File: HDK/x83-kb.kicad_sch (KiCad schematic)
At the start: 172 parts, among them U101 STM32F072C8Tx, U102 AMS1117-3.3

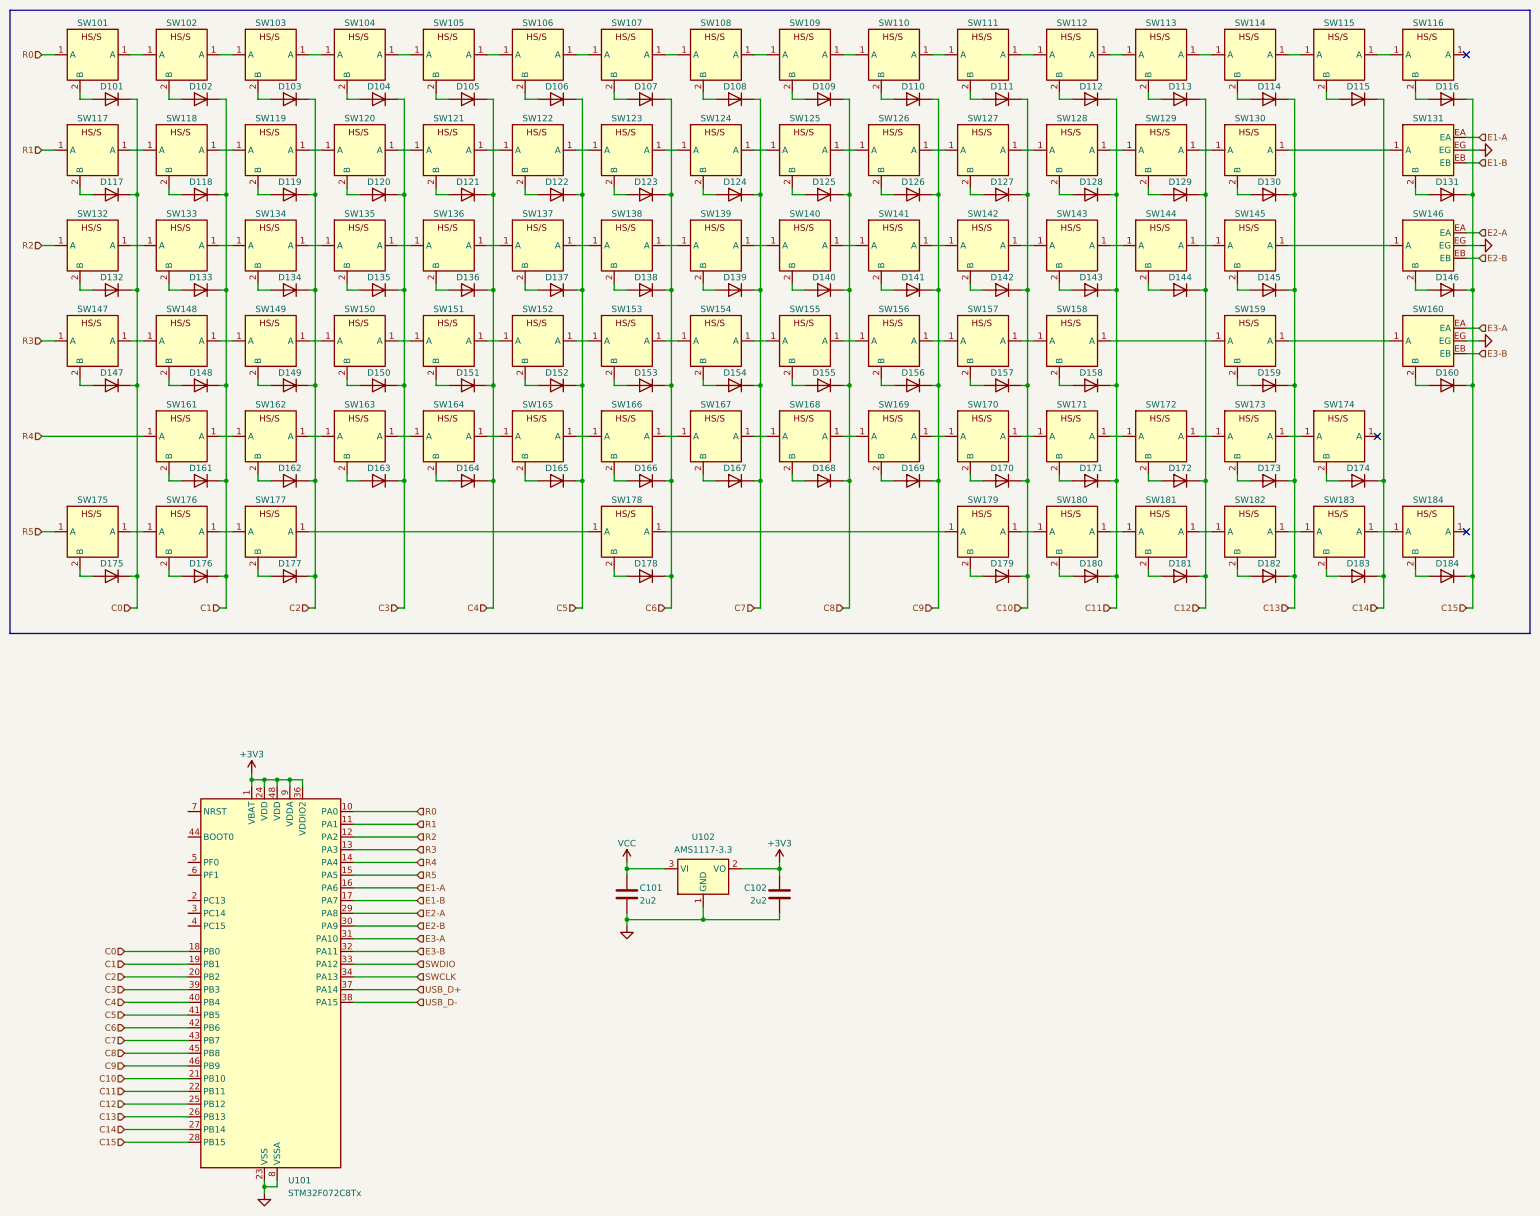
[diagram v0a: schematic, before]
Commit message: added rsc
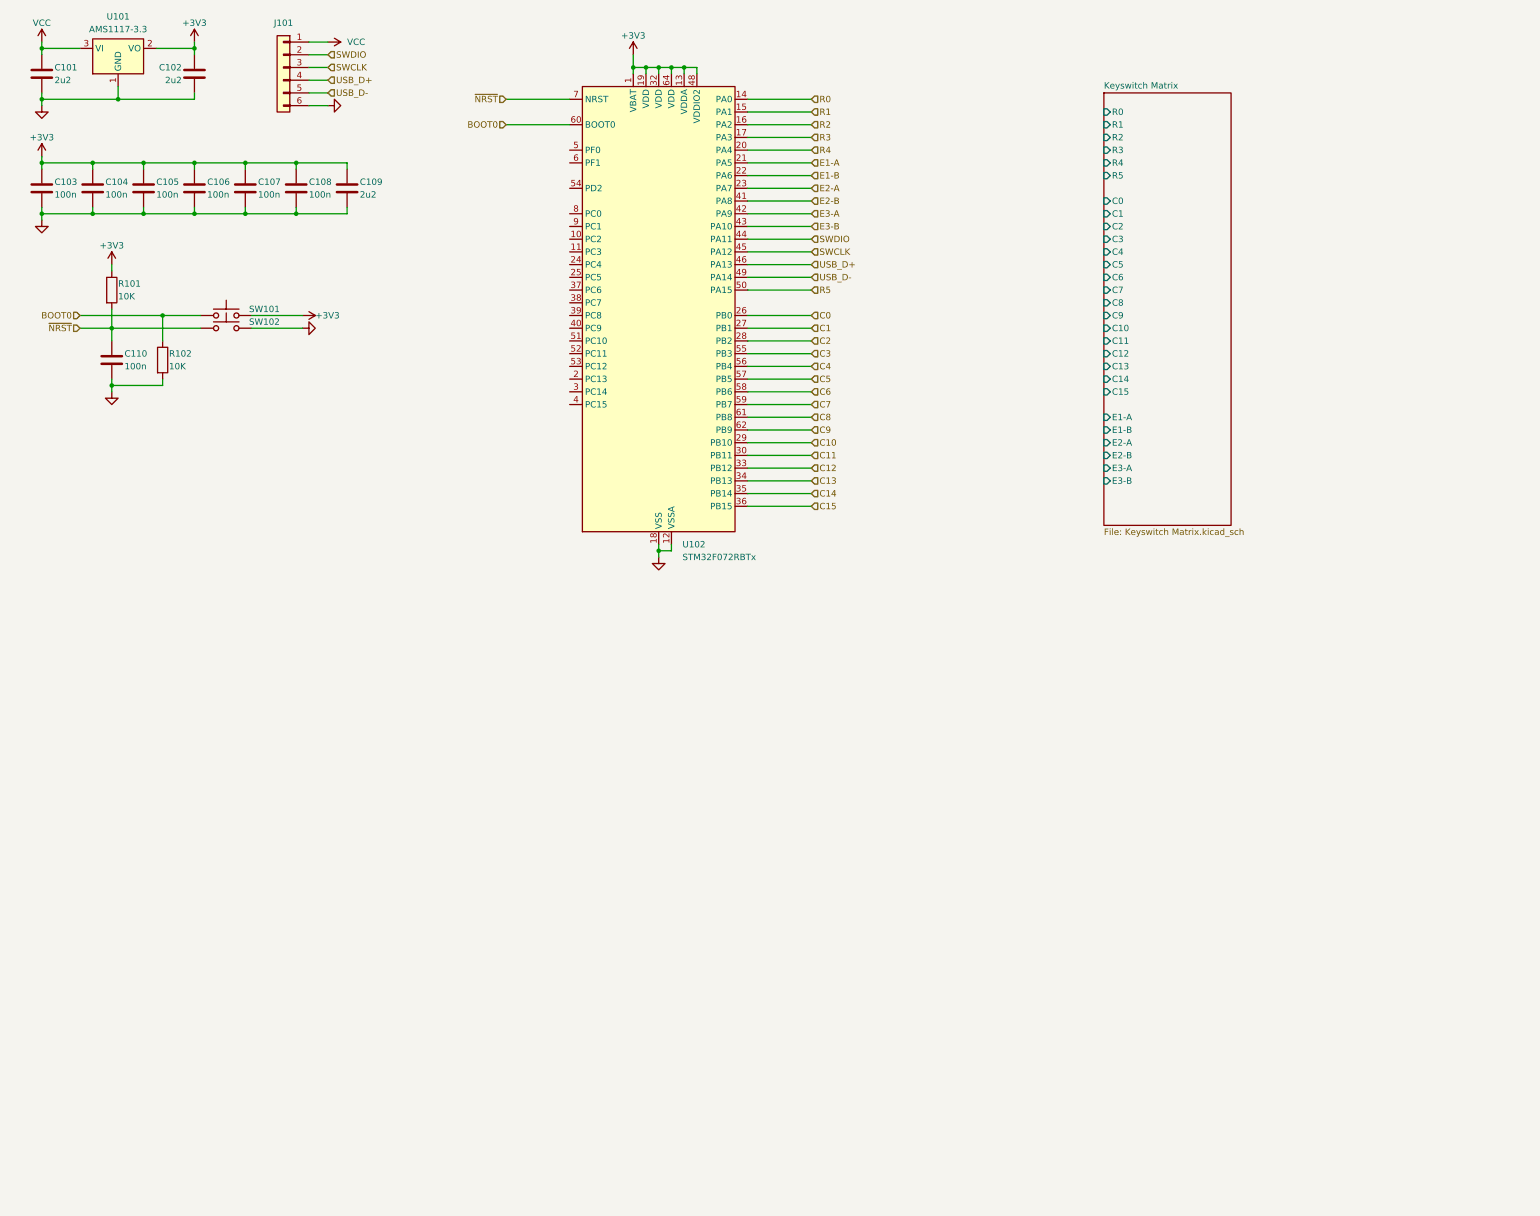
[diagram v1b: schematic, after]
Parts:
- removed D101, D102, D103, D104, D105, D106, D107, D108, D109, D110, D111, D112, D113, D114, D115, D116, D117, D118, D119, D120, D121, D122, D123, D124, D125, D126, D127, D128, D129, D130, D131, D132, D133, D134, D135, D136, D137, D138, D139, D140, D141, D142, D143, D144, D145, D146, D147, D148, D149, D150, D151, D152, D153, D154, D155, D156, D157, D158, D159, D160, D161, D162, D163, D164, D165, D166, D167, D168, D169, D170, D171, D172, D173, D174, D175, D176, D177, D178, D179, D180, D181, D182, D183, D184: D, symbol Device:D
- removed SW101, SW102, SW103, SW104, SW105, SW106, SW107, SW108, SW109, SW110, SW111, SW112, SW113, SW114, SW115, SW116, SW117, SW118, SW119, SW120, SW121, SW122, SW123, SW124, SW125, SW126, SW127, SW128, SW129, SW130, SW132, SW133, SW134, SW135, SW136, SW137, SW138, SW139, SW140, SW141, SW142, SW143, SW144, SW145, SW147, SW148, SW149, SW150, SW151, SW152, SW153, SW154, SW155, SW156, SW157, SW158, SW159, SW161, SW162, SW163, SW164, SW165, SW166, SW167, SW168, SW169, SW170, SW171, SW172, SW173, SW174, SW175, SW176, SW177, SW178, SW179, SW180, SW181, SW182, SW183, SW184: ~, symbol sckb-parts:HS/S-keyswitch
- removed SW131, SW146, SW160: ~, symbol sckb-parts:S-Keyswitch/ Rotary Encoder
- removed U101: STM32F072C8Tx, Package_QFP:LQFP-48_7x7mm_P0.5mm, symbol MCU_ST_STM32F0:STM32F072C8Tx
- removed U102: AMS1117-3.3, Package_TO_SOT_SMD:SOT-223-3_TabPin2, symbol Regulator_Linear:AMS1117-3.3
- added C103, C104, C105, C106, C107, C108, C110: 100n, Capacitor_SMD:C_0603_1608Metric, symbol Device:C
- added C109: 2u2, Capacitor_SMD:C_0805_2012Metric, symbol Device:C
- added J101: Conn_01x06, symbol Connector_Generic:Conn_01x06
- added R101, R102: 10K, Resistor_SMD:R_0603_1608Metric, symbol Device:R
- added SW101, SW102: SW_Push, symbol Switch:SW_Push
- added U101: AMS1117-3.3, Package_TO_SOT_SMD:SOT-223-3_TabPin2, symbol Regulator_Linear:AMS1117-3.3
- added U102: STM32F072RBTx, Package_QFP:LQFP-64_10x10mm_P0.5mm, symbol MCU_ST_STM32F0:STM32F072RBTx
- C101, C102: footprint (none) -> Capacitor_SMD:C_0805_2012Metric
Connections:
- net +3V3: now also C103.1, C104.1, C105.1, C106.1, C107.1, C108.1, C109.1, R101.1, SW101.2, U101.2 (VO), U102.1 (VBAT), U102.13 (VDDA), U102.19 (VDD), U102.32 (VDD), U102.48 (VDDIO2), U102.64 (VDD)
- net C0: now also U102.26 (PB0)
- net C1: now also U102.27 (PB1)
- net C10: now also U102.29 (PB10)
- net C11: now also U102.30 (PB11)
- net C12: now also U102.33 (PB12)
- net C13: now also U102.34 (PB13)
- net C14: now also U102.35 (PB14)
- net C15: now also U102.36 (PB15)
- net C2: now also U102.28 (PB2)
- net C3: now also U102.55 (PB3)
- net C4: now also U102.56 (PB4)
- net C5: now also U102.57 (PB5)
- net C6: now also U102.58 (PB6)
- net C7: now also U102.59 (PB7)
- net C8: now also U102.61 (PB8)
- net C9: now also U102.62 (PB9)
- net E1-A: now also U102.21 (PA5)
- net E1-B: now also U102.22 (PA6)
- net E2-A: now also U102.23 (PA7)
- net E2-B: now also U102.41 (PA8)
- net E3-A: now also U102.42 (PA9)
- net E3-B: now also U102.43 (PA10)
- net GND: now also C103.2, C104.2, C105.2, C106.2, C107.2, C108.2, C109.2, C110.2, J101.6 (Pin_6), R102.2, SW102.2, U101.1 (GND), U102.12 (VSSA), U102.18 (VSS), U102.31 (VSS), U102.47 (VSS), U102.63 (VSS)
- net R0: now also U102.14 (PA0)
- net R1: now also U102.15 (PA1)
- net R2: now also U102.16 (PA2)
- net R3: now also U102.17 (PA3)
- net R4: now also U102.20 (PA4)
- net R5: now also U102.50 (PA15)
- net SWCLK: now also J101.3 (Pin_3), U102.45 (PA12)
- net SWDIO: now also J101.2 (Pin_2), U102.44 (PA11)
- net USB_D+: now also J101.4 (Pin_4), U102.46 (PA13)
- net USB_D-: now also J101.5 (Pin_5), U102.49 (PA14)
- net VCC: now also J101.1 (Pin_1), U101.3 (VI)
- new net BOOT0: R102.1, SW101.1, U102.60 (BOOT0)
- new net ~{NRST}: C110.1, R101.2, SW102.1, U102.7 (NRST)
- no-connect marks 3 -> 0
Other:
- added sheet Keyswitch Matrix (Keyswitch Matrix.kicad_sch)
